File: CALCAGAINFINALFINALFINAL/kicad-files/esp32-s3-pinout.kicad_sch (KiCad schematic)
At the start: 13 parts, among them J1 Conn_01x11_Socket, J3 Micro_SD_Card, U8 ESP32-S3-WROOM-1

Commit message: dude this bitch ass project is the fucking boulder of sisyphus omfg ima genuinely kms at this rate if this iteration doesnt work ima genuinely kms like acutal this one is bare esp32 s3 with a diy antenna and crystal like dude what the actual fuck man ima genuinely dei. FINAL FINAL FINAL FINAL ITS GOT THE FUCKING BARE CHIPS FOR DAMN NEAR EVERYTHING DEAR MASS PRODUCED CHINK FACTORY GODS LET THIS THROUGH WITHOUT CAUSING A RUCKUS AND CHARGING LIKE $90 FOR 14 BUCKS OF PARTS AMEN
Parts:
- removed J1: Conn_01x11_Socket, Connector_JST:JST_EH_B11B-EH-A_1x11_P2.50mm_Vertical, symbol Connector:Conn_01x11_Socket
- removed U8: ESP32-S3-WROOM-1, RF_Module:ESP32-S3-WROOM-1, symbol RF_Module:ESP32-S3-WROOM-1
- added U1: ESP32-S3, Package_DFN_QFN:QFN-56-1EP_7x7mm_P0.4mm_EP4x4mm, symbol MCU_Espressif:ESP32-S3
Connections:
- net D+: now also U1.26 (GPIO20/USB_D+)
- net D-: now also U1.25 (GPIO19/USB_D-)
- net GND: now also U1.57 (GND)
- new net: U1.2 (VDD3P3), U1.3 (VDD3P3)
- new net: U1.55 (VDDA), U1.56 (VDDA)
- no-connect marks 25 -> 30
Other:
- note added: "==================================================================== ILI9341 40-PIN DISPLAY TO ESP32-S3 WROOM-1 WIRING LOG (4-WIRE SPI) ==================================================================== [POWER & GROUND] -------------------------------------------------------------------- Display Pin 5 (GND) --> Connect to GND Display Pin 6 (IOVCC) --> Connect to 3.3V Power Rail Display Pin 16 (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"
- note removed: "11-pin breakout has spi and i2c with extra pin wired for TX"
- note removed: "================================ J1 11-PIN EXPANSION PORT NOTES ================================ PINOUT MAPPING: - P1: GND | P7: MISO (IO14) [SPI Shared] - P2: 3V3 | P8: SCK (IO12) [SPI Shared] - P3: 5V (VBUS) | P9: CS1 (IO15) [Dedicated] - P4: SDA (IO7) | P10: IRQ (IO16) [Dedicated] - P5: SCL (IO6) | P11: TX (IO8) [Dedicated] - P6: MOSI(IO13) DESIGN & COEXISTENCE RULES: - SPI: Shares MOSI/SCK wi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"
- note removed: "pin header for extra accessories and whatnot"

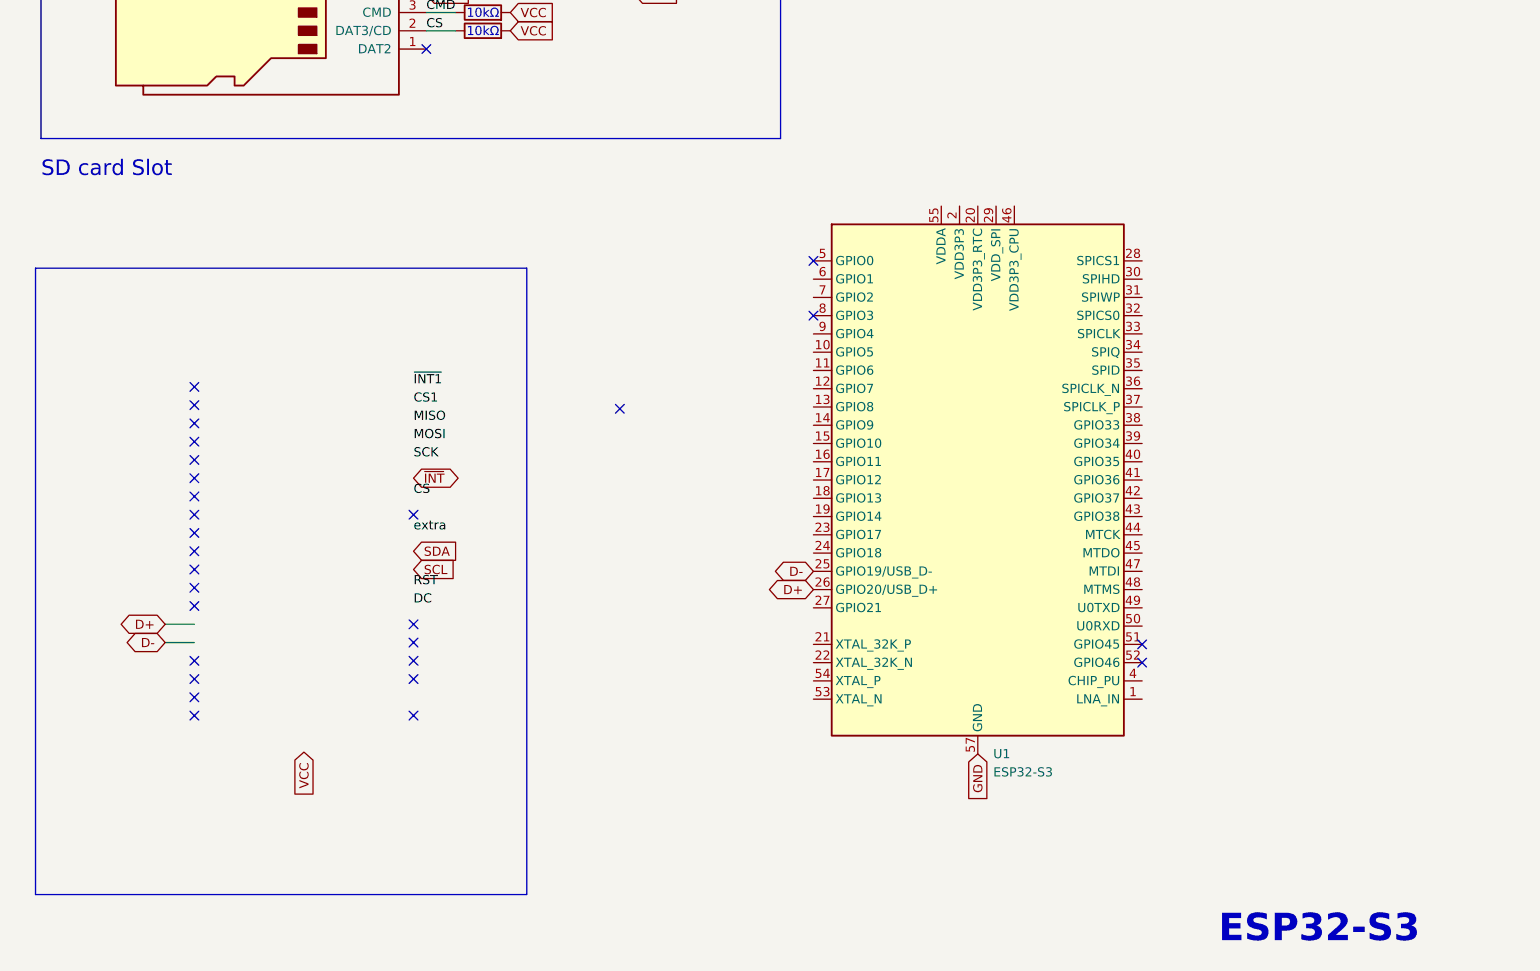
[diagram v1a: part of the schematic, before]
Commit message: I reckon its all done now. need to doucble check all pin assignments tomorrow and then add camera then order everything. we might lowkirkenuinely launch this shit chat
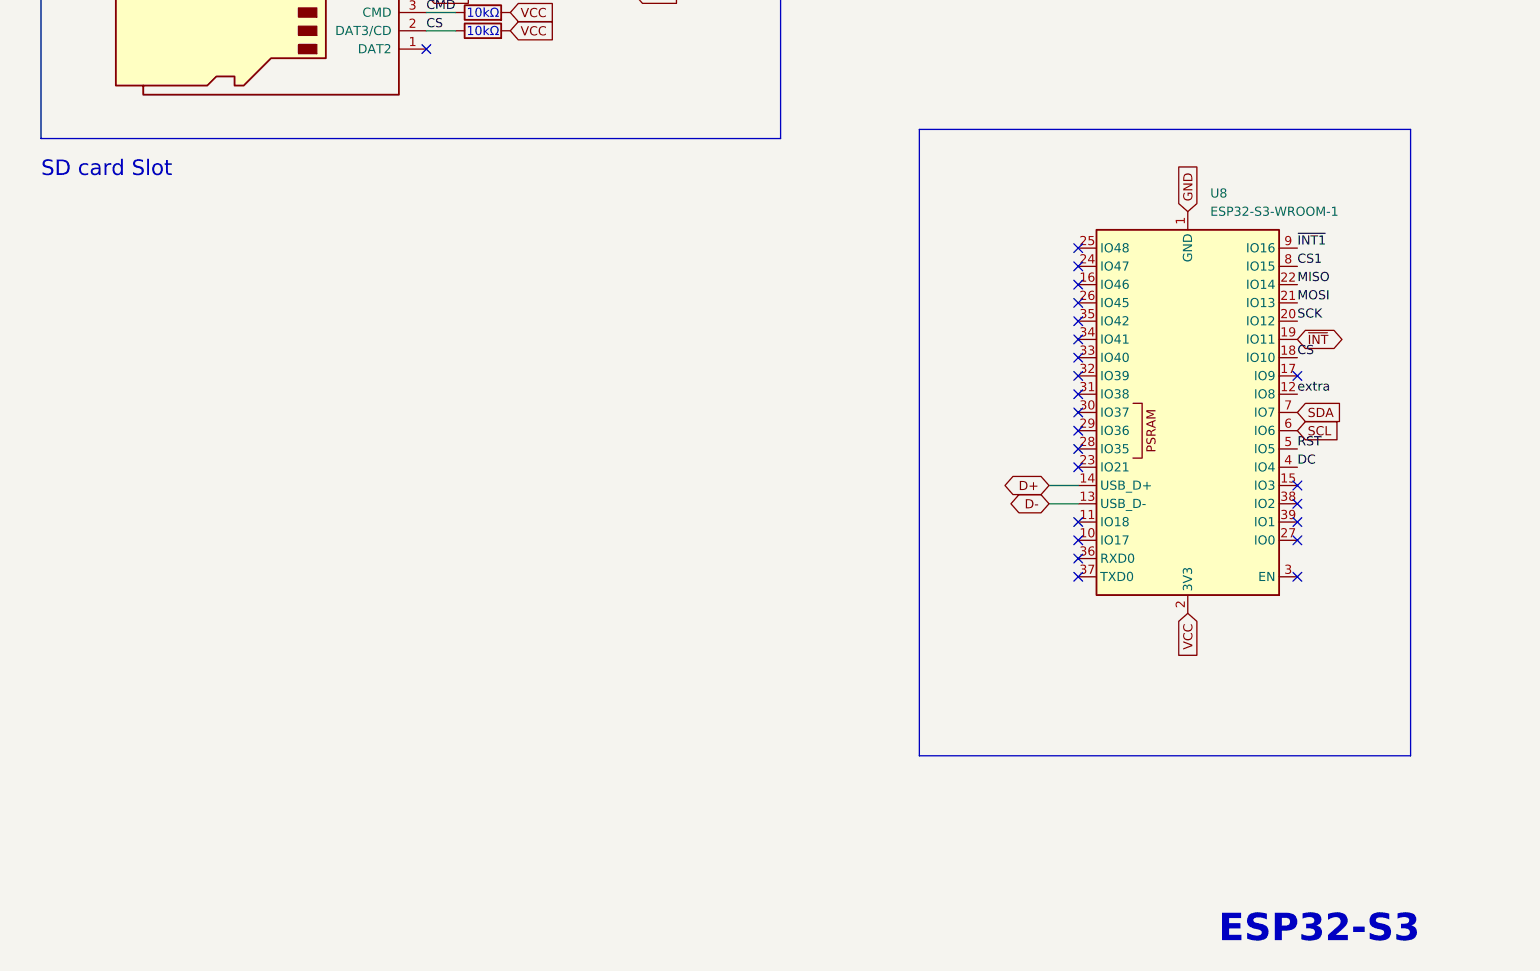
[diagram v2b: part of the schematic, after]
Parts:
- removed U1: ESP32-S3, Package_DFN_QFN:QFN-56-1EP_7x7mm_P0.4mm_EP4x4mm, symbol MCU_Espressif:ESP32-S3
- added U8: ESP32-S3-WROOM-1, RF_Module:ESP32-S3-WROOM-1, symbol RF_Module:ESP32-S3-WROOM-1
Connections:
- net CS: now also U8.18 (IO10)
- net CS1: now also U8.8 (IO15)
- net D+: now also U8.14 (USB_D+)
- net D-: now also U8.13 (USB_D-)
- net DC: now also U8.4 (IO4)
- net GND: now also U8.1 (GND), U8.40 (GND), U8.41 (GND)
- net MISO: now also U8.22 (IO14)
- net MOSI: now also U8.21 (IO13)
- net RST: now also U8.5 (IO5)
- net SCK: now also U8.20 (IO12)
- net SCL: now also U8.6 (IO6)
- net SDA: now also U8.7 (IO7)
- net VCC: now also U8.2 (3V3)
- net extra: now also U8.12 (IO8)
- net ~{INT1}: now also U8.9 (IO16)
- net ~{INT}: now also U8.19 (IO11)
- no-connect marks 30 -> 25
